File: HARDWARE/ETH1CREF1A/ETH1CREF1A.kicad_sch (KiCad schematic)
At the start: 0 parts

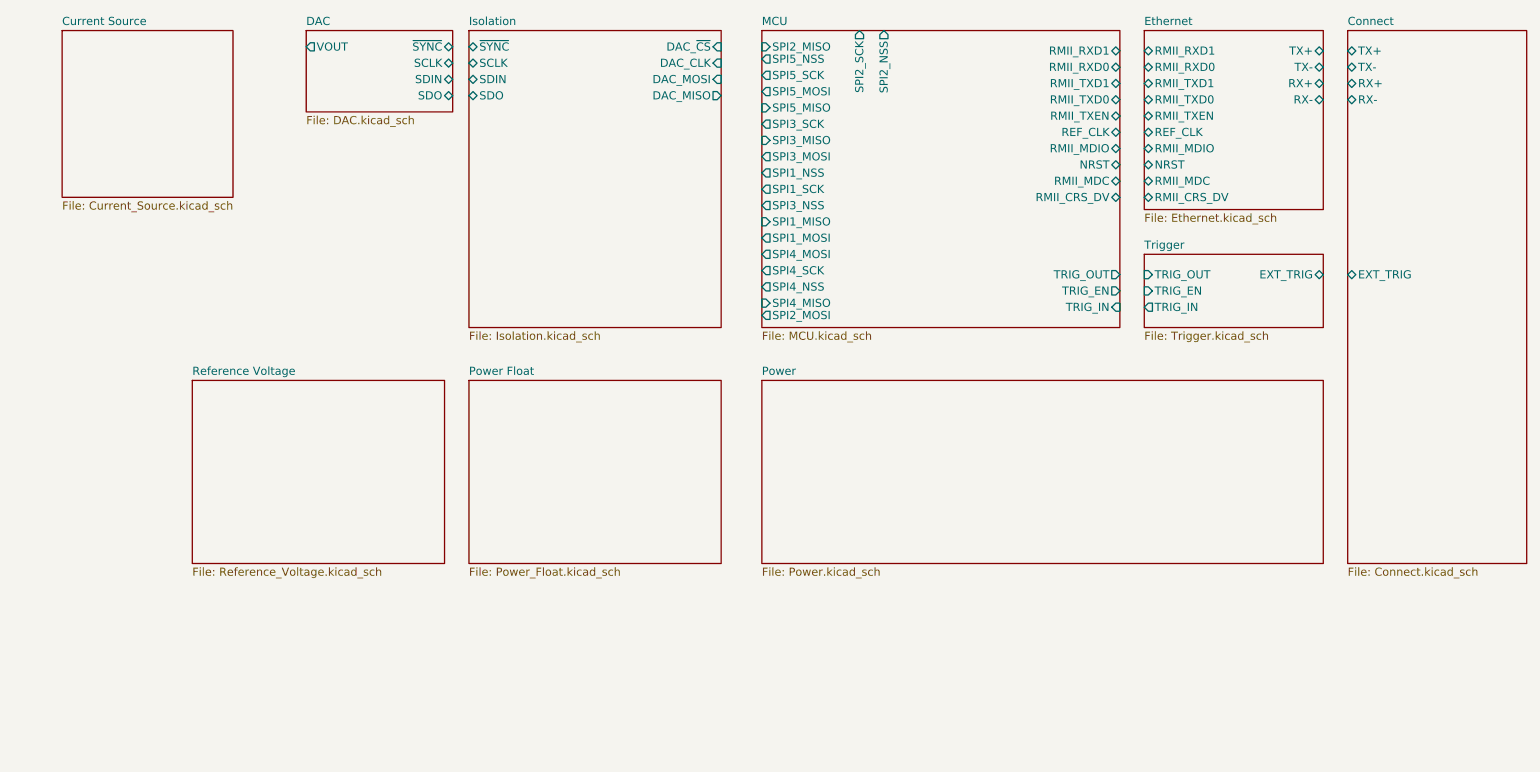
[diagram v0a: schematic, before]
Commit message: Hardware
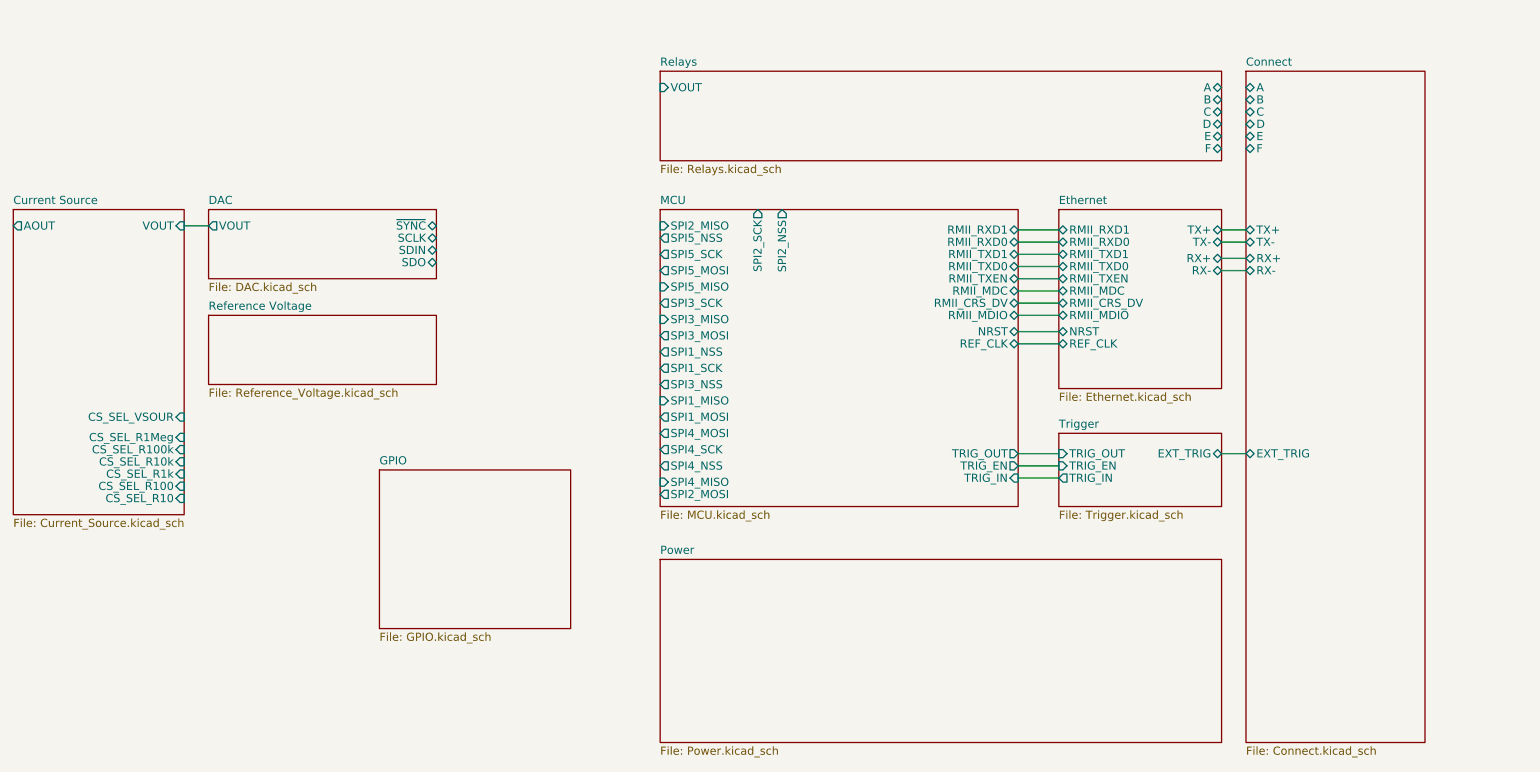
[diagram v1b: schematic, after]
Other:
- removed sheet Isolation
- removed sheet Power Float
- added sheet GPIO (GPIO.kicad_sch)
- added sheet Relays (Relays.kicad_sch)
- sheet Connect ports: added A, B, C, D, E, F; removed none
- sheet Current Source ports: added AOUT, CS_SEL_R10, CS_SEL_R100, CS_SEL_R100k, CS_SEL_R10k, CS_SEL_R1Meg, CS_SEL_R1k, CS_SEL_VSOUR, VOUT; removed none
- title: (none) -> ETH1CREF1A

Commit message: Hardware
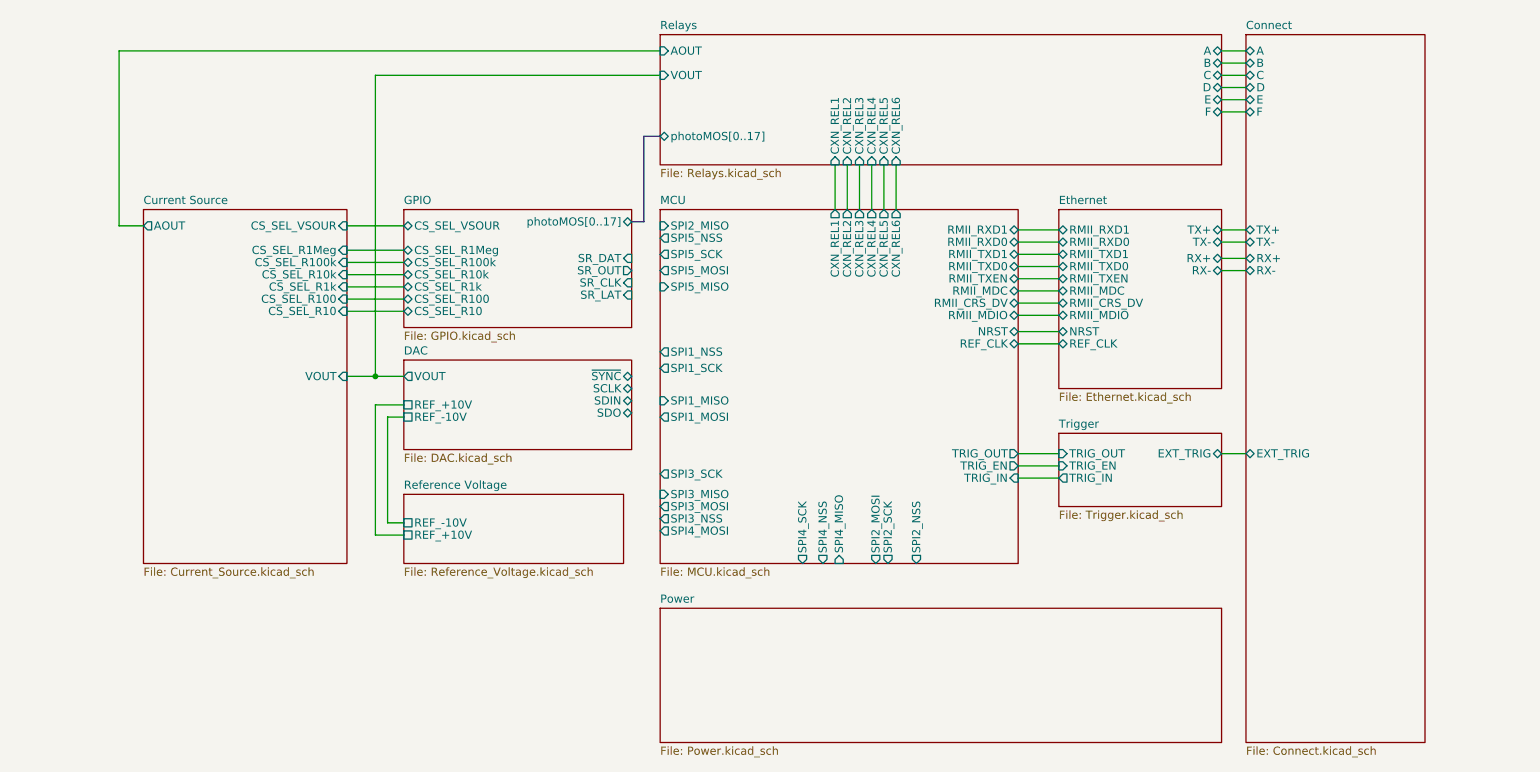
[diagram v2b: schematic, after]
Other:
- sheet DAC ports: added REF_+10V, REF_-10V; removed none
- sheet GPIO ports: added CS_SEL_R10, CS_SEL_R100, CS_SEL_R100k, CS_SEL_R10k, CS_SEL_R1Meg, CS_SEL_R1k, CS_SEL_VSOUR, SR_CLK, SR_DAT, SR_LAT, SR_OUT, photoMOS[0..17]; removed none
- sheet MCU ports: added CXN_REL1, CXN_REL2, CXN_REL3, CXN_REL4, CXN_REL5, CXN_REL6; removed none
- sheet Reference Voltage ports: added REF_+10V, REF_-10V; removed none
- sheet Relays ports: added AOUT, CXN_REL1, CXN_REL2, CXN_REL3, CXN_REL4, CXN_REL5, CXN_REL6, photoMOS[0..17]; removed none
